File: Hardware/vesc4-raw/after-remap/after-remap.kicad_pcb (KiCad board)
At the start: 4 copper layers, 38.5 x 65 mm, 127 parts, among them K1 SERVO, P1 HALL/Encoder, P101 CANBUS, P2 SWD, P3 PWR_COMM, P4 IN+, P5 IN-, P6 MOTOR1, P7 MOTOR2, P9 MOTOR3, Q1 IPT007N06NATMA1, Q2 IPT007N06NATMA1, Q3 IPT007N06NATMA1, Q4 IPT007N06NATMA1, Q5 IPT007N06NATMA1, Q6 IPT007N06NATMA1, U1 STM32F40X_LQFP64, U2 TC2117, U3 DRV8302, U401 SN65HVD232, X1 MINI-USB-SHIELD-32005-201, X2 8MHz 10ppm

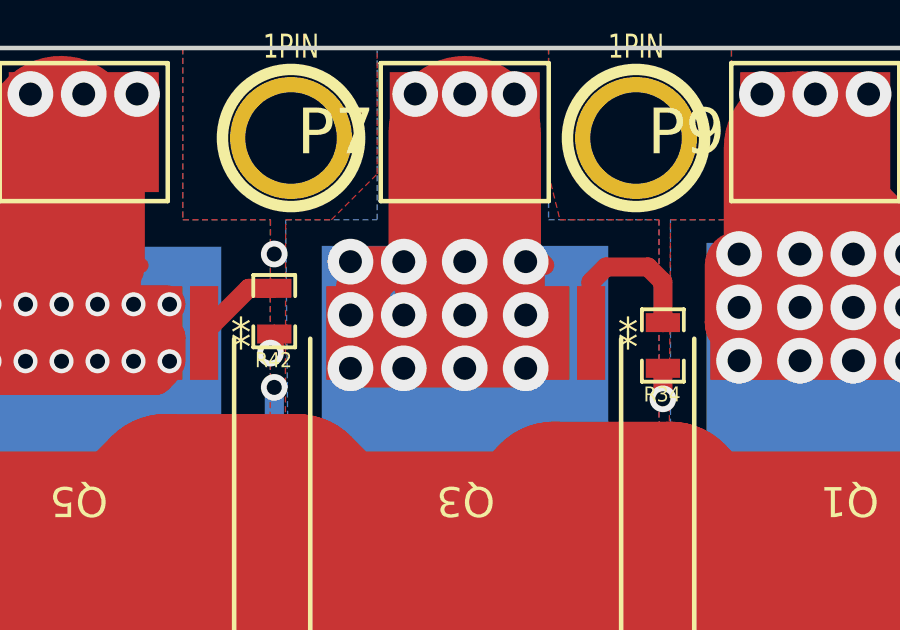
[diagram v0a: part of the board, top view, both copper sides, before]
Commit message: change phase tengah
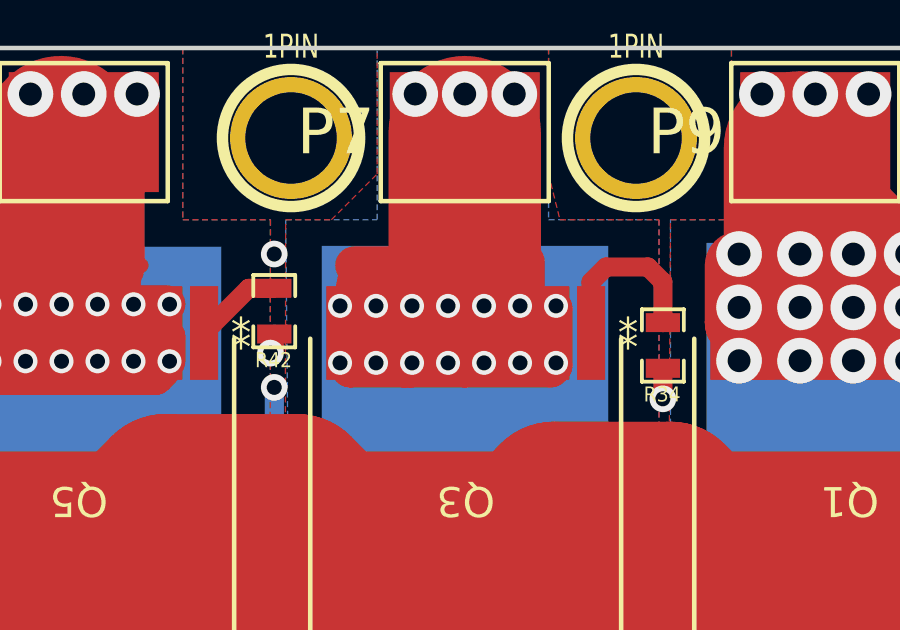
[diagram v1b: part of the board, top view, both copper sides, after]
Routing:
- net /Power MOSFETS/Q3-s_Q4-d: track 145.0 -> 145.9 mm, vias 17 -> 19

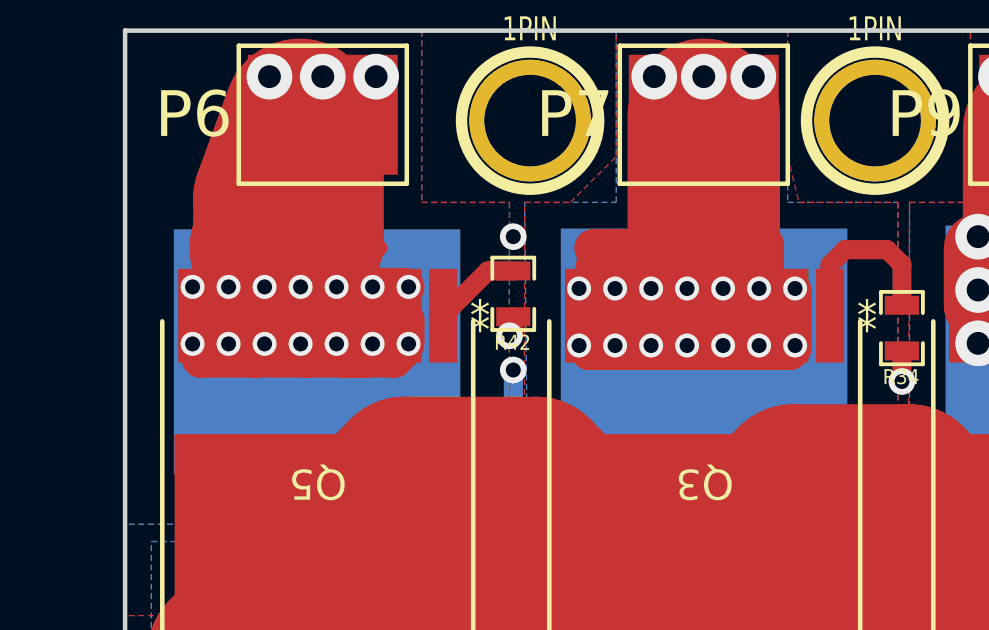
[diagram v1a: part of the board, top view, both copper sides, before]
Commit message: pindahin via untuk perbanyak contact
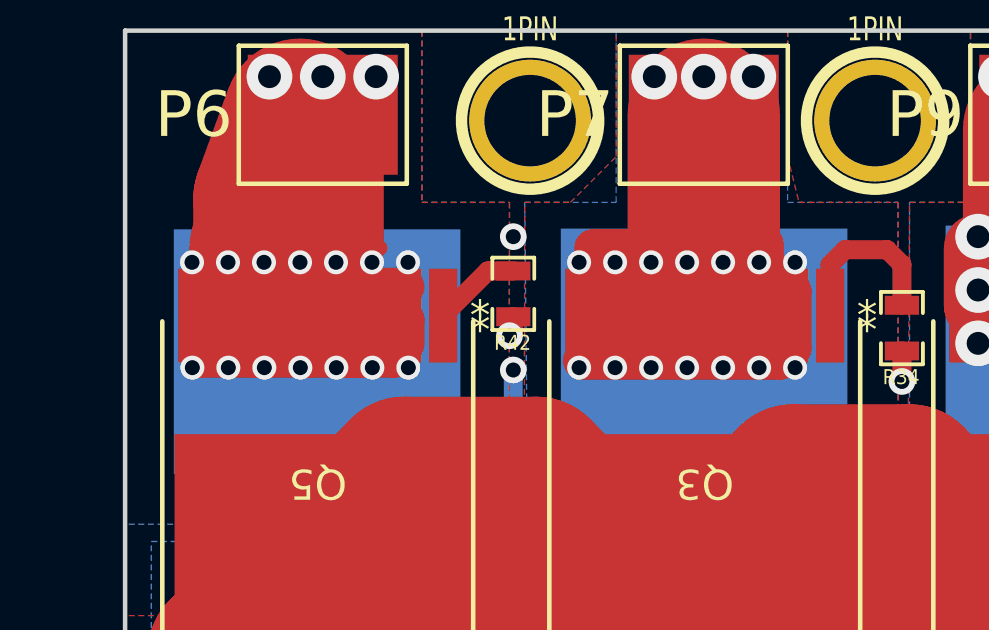
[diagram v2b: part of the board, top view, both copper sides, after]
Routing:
- net /Power MOSFETS/Q3-s_Q4-d: track 145.9 -> 153.3 mm
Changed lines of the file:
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@@
 	(segment
 		(start 104.394 91.694)
-		(end 105.537509 92.837509)
+		(end 104.4 91.7)
 		(width 0.635)
 		(layer "In1.Cu")
@@
 	)
 	(segment
-		(start 105.537509 92.837509)
-		(end 105.537509 101.941532)
+		(start 104.4 93.4)
+		(end 105.537509 94.537509)
 		(width 0.635)
 		(layer "In1.Cu")
@@
 	)
 	(segment
-		(start 105.537509 101.941532)
+		(start 105.537509 94.537509)
 		(end 105.537509 102.507217)
 		(width 0.635)
@@
 	)
 	(segment
+		(start 104.4 91.7)
+		(end 104.4 93.4)
+		(width 0.635)
+		(layer "In1.Cu")
+		(net 17)
+	)
+	(segment
 		(start 102.9966 112.845202)
 		(end 102.596601 113.245201)
@@
 	)
 	(segment
-		(start 100.7441 88.68528)
-		(end 100.7441 90.58528)
+		(start 100.7441 90.58528)
+		(end 100.65138 90.678)
 		(width 1.27)
 		(layer "F.Cu")
@@
 	)
 	(segment
-		(start 99.0186 88.9)
-		(end 100.52938 88.9)
-		(width 1.27)
-		(layer "F.Cu")
-		(net 68)
-	)
-	(segment
 		(start 97.79 82.804)
 		(end 98.171 82.804)
@@
 	)
 	(segment
+		(start 100.52938 88.9)
+		(end 100.7441 88.68528)
+		(width 1.27)
+		(layer "F.Cu")
+		(net 68)
+	)
+	(segment
 		(start 102.489 108.839)
 		(end 102.489 105.41)
@@
 	)
 	(segment
-		(start 100.7441 90.58528)
-		(end 100.65138 90.678)
+		(start 98.4186 89.5)
+		(end 99.0186 88.9)
 		(width 1.27)
 		(layer "F.Cu")
@@
 	)
 	(segment
-		(start 100.52938 88.9)
-		(end 100.7441 88.68528)
+		(start 100.65138 90.678)
+		(end 100.32938 91)
 		(width 1.27)
 		(layer "F.Cu")
@@
 	)
 	(segment
+		(start 100.7441 88.68528)
+		(end 100.7441 90.58528)
+		(width 1.27)
+		(layer "F.Cu")
+		(net 68)
+	)
+	(segment
 		(start 102.489 104.5337)
 		(end 103.790707 103.231993)
@@
 	)
 	(segment
+		(start 100.32938 91)
+		(end 93.732 91)
+		(width 1.27)
+		(layer "F.Cu")
+		(net 68)
+	)
+	(segment
 		(start 95.758 90.678)
 		(end 97.79 90.678)
@@
 	)
 	(segment
-		(start 98.4186 89.5)
-		(end 99.0186 88.9)
-		(width 1.27)
-		(layer "F.Cu")
-		(net 68)
-	)
-	(segment
 		(start 95.758 90.678)
 		(end 95.758 88.9)
@@
 	)
 	(segment
+		(start 99.0186 88.9)
+		(end 100.52938 88.9)
+		(width 1.27)
+		(layer "F.Cu")
+		(net 68)
+	)
+	(segment
 		(start 102.730299 110.730027)
 		(end 102.730299 109.080299)
@@
 	)
 	(via
-		(at 96.033048 90.496332)
+		(at 96.033048 91.234337)
 		(size 0.8)
 		(drill 0.5)
@@
 	)
 	(via
-		(at 100.833048 88.596332)
+		(at 100.833048 87.72272)
 		(size 0.8)
 		(drill 0.5)
@@
 	)
 	(via
-		(at 96.033048 88.596332)
+		(at 96.033048 87.72272)
 		(size 0.8)
 		(drill 0.5)
@@
 	)
 	(via
-		(at 93.633048 88.596332)
+		(at 93.633048 87.72272)
 		(size 0.8)
 		(drill 0.5)
@@
 	)
 	(via
-		(at 94.833048 90.496332)
+		(at 94.833048 91.234337)
 		(size 0.8)
 		(drill 0.5)
@@
 	)
 	(via
-		(at 98.433048 90.496332)
+		(at 98.433048 91.234337)
 		(size 0.8)
 		(drill 0.5)
@@
 	)
 	(via
-		(at 99.633048 90.496332)
+		(at 99.633048 91.234337)
 		(size 0.8)
 		(drill 0.5)
@@
 	)
 	(via
-		(at 93.633048 90.496332)
+		(at 93.633048 91.234337)
 		(size 0.8)
 		(drill 0.5)
@@
 	)
 	(via
-		(at 94.833048 88.596332)
+		(at 94.833048 87.72272)
 		(size 0.8)
 		(drill 0.5)
@@
 	)
 	(via
-		(at 97.233048 88.596332)
+		(at 97.233048 87.72272)
 		(size 0.8)
 		(drill 0.5)
@@
 	)
 	(via
-		(at 97.233048 90.496332)
+		(at 97.233048 91.234337)
 		(size 0.8)
 		(drill 0.5)
@@
 	)
 	(via
-		(at 98.433048 88.596332)
+		(at 98.433048 87.72272)
 		(size 0.8)
 		(drill 0.5)
@@
 	)
 	(via
-		(at 99.633048 88.596332)
+		(at 99.633048 87.72272)
 		(size 0.8)
 		(drill 0.5)
@@
 	)
 	(via
-		(at 100.833048 90.496332)
+		(at 100.833048 91.234337)
 		(size 0.8)
 		(drill 0.5)
@@
 	)
 	(segment
+		(start 102.010328 88.9)
+		(end 103.378 88.9)
+		(width 0.635)
+		(layer "In1.Cu")
+		(net 68)
+	)
+	(segment
 		(start 97.396311 111.391689)
 		(end 104.406689 111.391689)
@@
 	)
 	(segment
+		(start 107.1 102.691825)
+		(end 106.159825 103.632)
+		(width 0.635)
+		(layer "In1.Cu")
+		(net 68)
+	)
+	(segment
 		(start 104.406689 111.391689)
 		(end 106.172 113.157)
@@
 	)
 	(segment
-		(start 103.378 88.9)
-		(end 107.1 92.622)
-		(width 0.635)
+		(start 105.994139 104.031999)
+		(end 105.59414 103.632)
+		(width 0.254)
 		(layer "In1.Cu")
 		(net 68)
 	)
 	(segment
-		(start 107.1 102.691825)
-		(end 106.159825 103.632)
-		(width 0.635)
+		(start 91.2 123.6)
+		(end 90.800001 123.200001)
+		(width 0.254)
 		(layer "In1.Cu")
 		(net 68)
 	)
 	(segment
-		(start 105.994139 104.031999)
-		(end 105.59414 103.632)
-		(width 0.254)
+		(start 105.5 93.1)
+		(end 107.1 94.7)
+		(width 0.635)
 		(layer "In1.Cu")
 		(net 68)
 	)
 	(segment
-		(start 91.2 123.6)
-		(end 90.800001 123.200001)
-		(width 0.254)
+		(start 99.633048 87.72272)
+		(end 100.833048 87.72272)
+		(width 0.635)
 		(layer "In1.Cu")
 		(net 68)
@@
 	)
 	(segment
-		(start 99.633048 88.596332)
-		(end 99.936716 88.9)
-		(width 0.635)
-		(layer "In1.Cu")
-		(net 68)
-	)
-	(segment
 		(start 106.159825 103.632)
 		(end 105.41 103.632)
@@
 	)
 	(segment
-		(start 107.1 92.622)
-		(end 107.1 102.691825)
+		(start 100.833048 87.72272)
+		(end 102.010328 88.9)
 		(width 0.635)
 		(layer "In1.Cu")
@@
 	)
 	(segment
-		(start 99.936716 88.9)
-		(end 103.378 88.9)
+		(start 105.5 91.022)
+		(end 105.5 93.1)
 		(width 0.635)
 		(layer "In1.Cu")
@@
 	)
 	(segment
+		(start 107.1 94.7)
+		(end 107.1 102.691825)
+		(width 0.635)
+		(layer "In1.Cu")
+		(net 68)
+	)
+	(segment
+		(start 103.378 88.9)
+		(end 105.5 91.022)
+		(width 0.635)
+		(layer "In1.Cu")
+		(net 68)
+	)
+	(segment
 		(start 83.312 85.598)
 		(end 83.312 87.122)
@@
 	)
 	(via
-		(at 86.749702 88.542327)
+		(at 86.730095 87.72272)
 		(size 0.8)
 		(drill 0.5)
@@
 	)
 	(via
-		(at 87.949702 88.542327)
+		(at 87.930095 87.72272)
 		(size 0.8)
 		(drill 0.5)
@@
 	)
 	(via
-		(at 84.349702 90.442327)
+		(at 84.341138 91.234337)
 		(size 0.8)
 		(drill 0.5)
@@
 	)
 	(via
-		(at 84.349702 88.542327)
+		(at 84.330095 87.72272)
 		(size 0.8)
 		(drill 0.5)
@@
 	)
 	(via
-		(at 81.949702 88.542327)
+		(at 81.930095 87.72272)
 		(size 0.8)
 		(drill 0.5)
@@
 	)
 	(via
-		(at 83.149702 88.542327)
+		(at 83.130095 87.72272)
 		(size 0.8)
 		(drill 0.5)
@@
 	)
 	(via
-		(at 85.549702 88.542327)
+		(at 85.530095 87.72272)
 		(size 0.8)
 		(drill 0.5)
@@
 	)
 	(via
-		(at 80.749702 90.442327)
+		(at 80.741138 91.234337)
 		(size 0.8)
 		(drill 0.5)
@@
 	)
 	(via
-		(at 81.949702 90.442327)
+		(at 81.941138 91.234337)
 		(size 0.8)
 		(drill 0.5)
@@
 	)
 	(via
-		(at 87.949702 90.442327)
+		(at 87.941138 91.234337)
 		(size 0.8)
 		(drill 0.5)
@@
 	)
 	(via
-		(at 86.749702 90.442327)
+		(at 86.741138 91.234337)
 		(size 0.8)
 		(drill 0.5)
@@
 	)
 	(via
-		(at 83.149702 90.442327)
+		(at 83.141138 91.234337)
 		(size 0.8)
 		(drill 0.5)
@@
 	)
 	(via
-		(at 85.549702 90.442327)
+		(at 85.541138 91.234337)
 		(size 0.8)
 		(drill 0.5)
@@
 	)
 	(via
-		(at 80.749702 88.542327)
+		(at 80.730095 87.72272)
 		(size 0.8)
 		(drill 0.5)

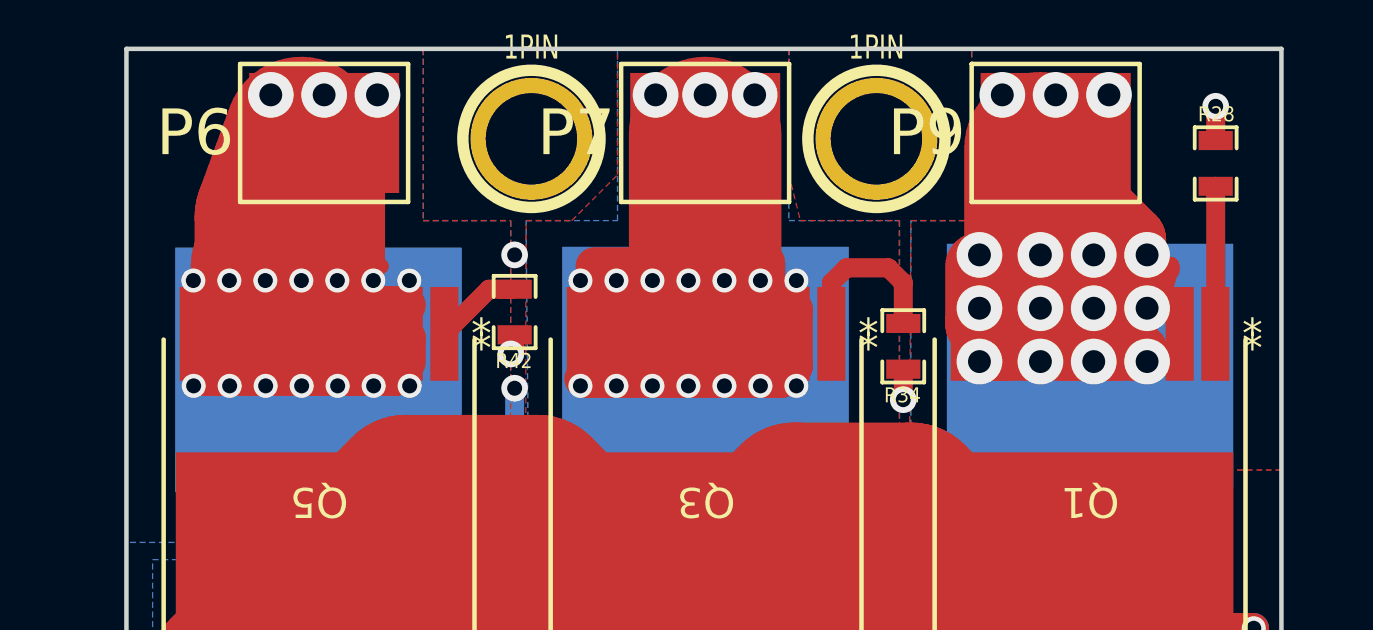
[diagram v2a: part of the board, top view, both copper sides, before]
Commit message: done changed via numpuk
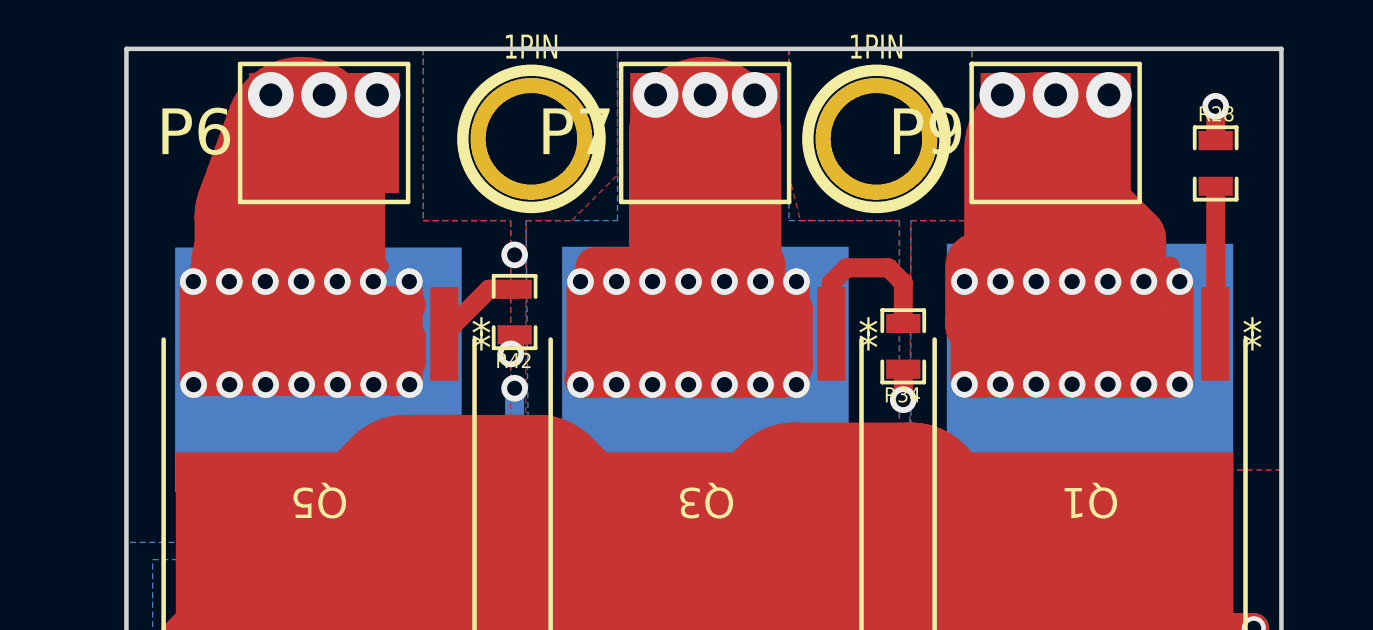
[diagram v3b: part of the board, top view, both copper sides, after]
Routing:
- net /Power MOSFETS/Q1-s_Q2-d: track 150.9 -> 159.1 mm, vias 17 -> 19
